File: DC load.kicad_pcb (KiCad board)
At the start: 2 copper layers, 33.3 x 44.4 mm, 27 parts, among them J1 CTL IN, J2 CTL OUT, J3 B+, J4 B-, M2 3.2mm, M3 3.2mm, Q1 IRFI540, U1 LM324

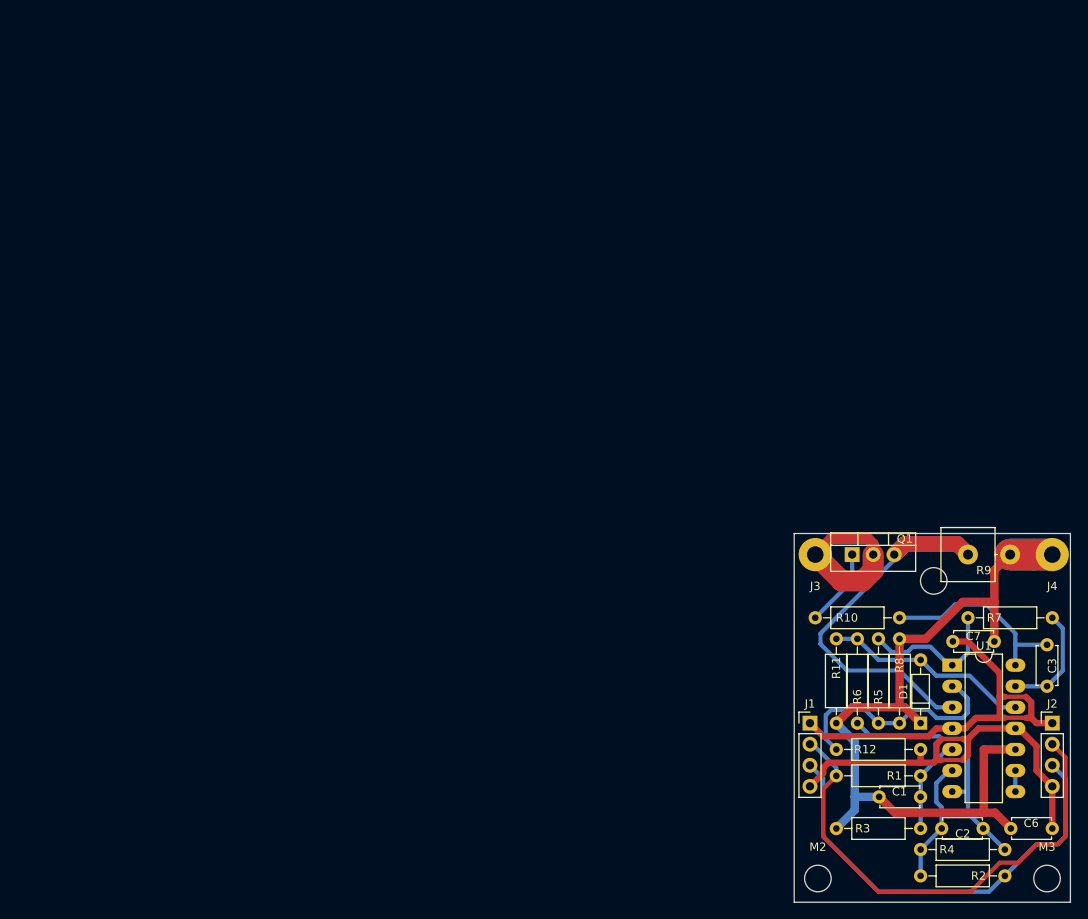
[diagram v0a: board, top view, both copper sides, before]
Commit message: Prepare for production
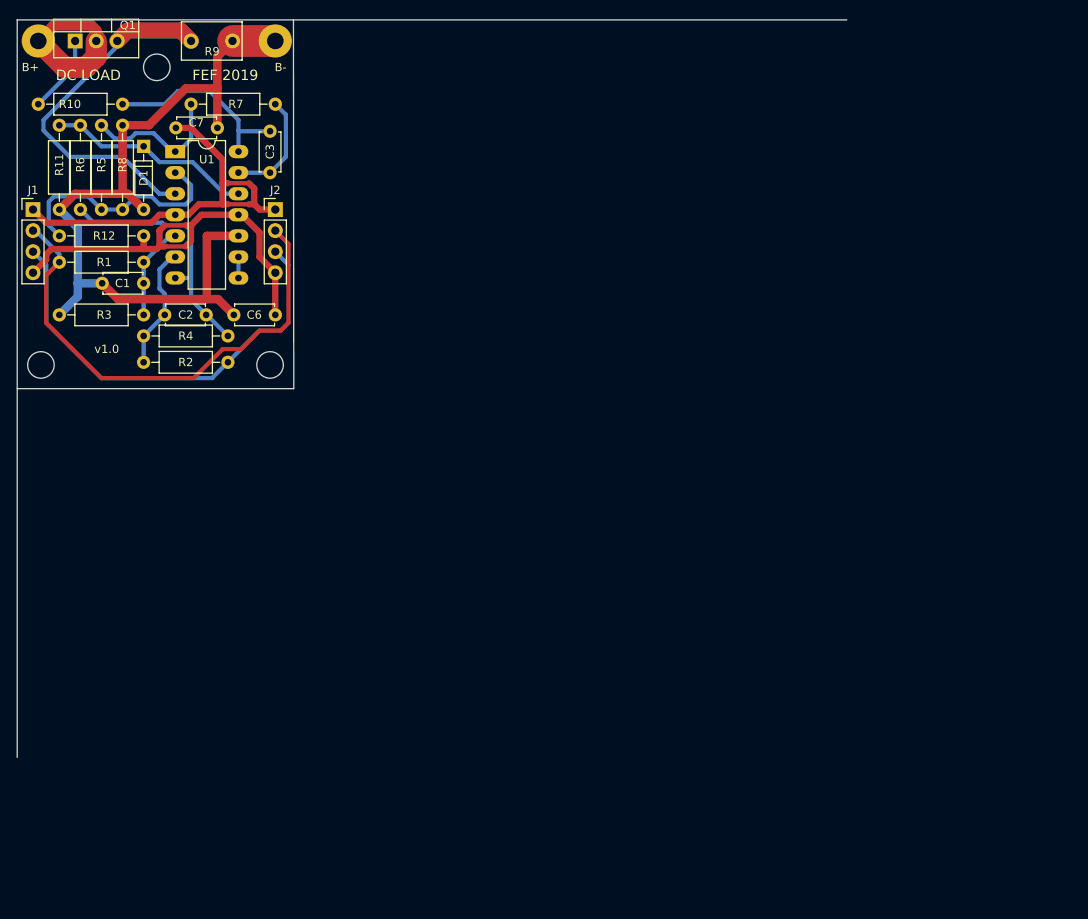
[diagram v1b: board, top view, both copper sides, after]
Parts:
- R9: footprint Resistors_THT:R_Axial_Power_L20.0mm_W6.4mm_P5.08mm_Vertical -> Capacitors_THT:C_Rect_L7.2mm_W4.5mm_P5.00mm_FKS2_FKP2_MKS2_MKP2
- moved D1 116.7 mm to (48.6, 48.6), turned to 270 degrees
- moved Q1 112.3 mm to (40.3, 35.9)
- moved R11 112.3 mm to (38.4, 56.2)
- moved R9 112.3 mm to (54.3, 35.9)
- moved B- 112.3 mm to (64.5, 35.9)
- moved C1 112.3 mm to (43.6, 65.1)
- moved C6 112.3 mm to (64.5, 68.9)
- moved J2 112.3 mm to (64.5, 56.2)
- moved R1 112.3 mm to (48.6, 62.5)
- moved R12 112.3 mm to (38.4, 59.4)
- moved R2 112.3 mm to (48.6, 74.6)
- moved R3 112.3 mm to (48.6, 68.9)
- moved R4 112.3 mm to (58.7, 71.4)
- moved R7 112.3 mm to (64.5, 43.5)
- moved U1 112.3 mm to (52.4, 49.2)
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- renumbered J3 to B+, J4 to B-, MP1 to M1
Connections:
- D1 pad 1: GND -> Net-(D1-Pad1)
- D1 pad 2: Net-(D1-Pad2) -> GND
- R11 pad 2: Net-(D1-Pad2) -> Net-(D1-Pad1)
- R6 pad 2: Net-(D1-Pad2) -> Net-(D1-Pad1)
- U1 pad 12: Net-(D1-Pad2) -> Net-(D1-Pad1)
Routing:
- net Net-(D1-Pad1): track 0.00 -> 25.4 mm
- net Net-(D1-Pad2): track 25.4 -> 0.00 mm
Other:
- board size 33.3 x 44.4 mm -> 100 x 88.9 mm
- board text added: "DC LOAD"
- board text added: "FEF 2019"
- board text added: "v1.0"
